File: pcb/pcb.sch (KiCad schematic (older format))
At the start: 70 parts, among them SW1 SW_PUSH, SW10 SW_PUSH, SW11 SW_PUSH, SW12 SW_PUSH, SW13 SW_PUSH, SW14 SW_PUSH, SW15 SW_PUSH, SW16 SW_PUSH, SW17 SW_PUSH, SW18 SW_PUSH, SW19 SW_PUSH, SW2 SW_PUSH, SW20 SW_PUSH, SW21 SW_PUSH, SW22 SW_PUSH, SW23 SW_PUSH, SW24 SW_PUSH, SW25 SW_PUSH, SW26 SW_PUSH, SW27 SW_PUSH, SW28 SW_PUSH, SW29 SW_PUSH, SW3 SW_PUSH, SW30 SW_PUSH, SW31 SW_PUSH, SW32 SW_PUSH, SW33 Rotary_Encoder_Switch, SW34 SW_PUSH, SW4 SW_PUSH, SW5 SW_PUSH, SW6 SW_PUSH, SW7 SW_PUSH, SW8 SW_PUSH, SW9 SW_PUSH, U1 ProMicro

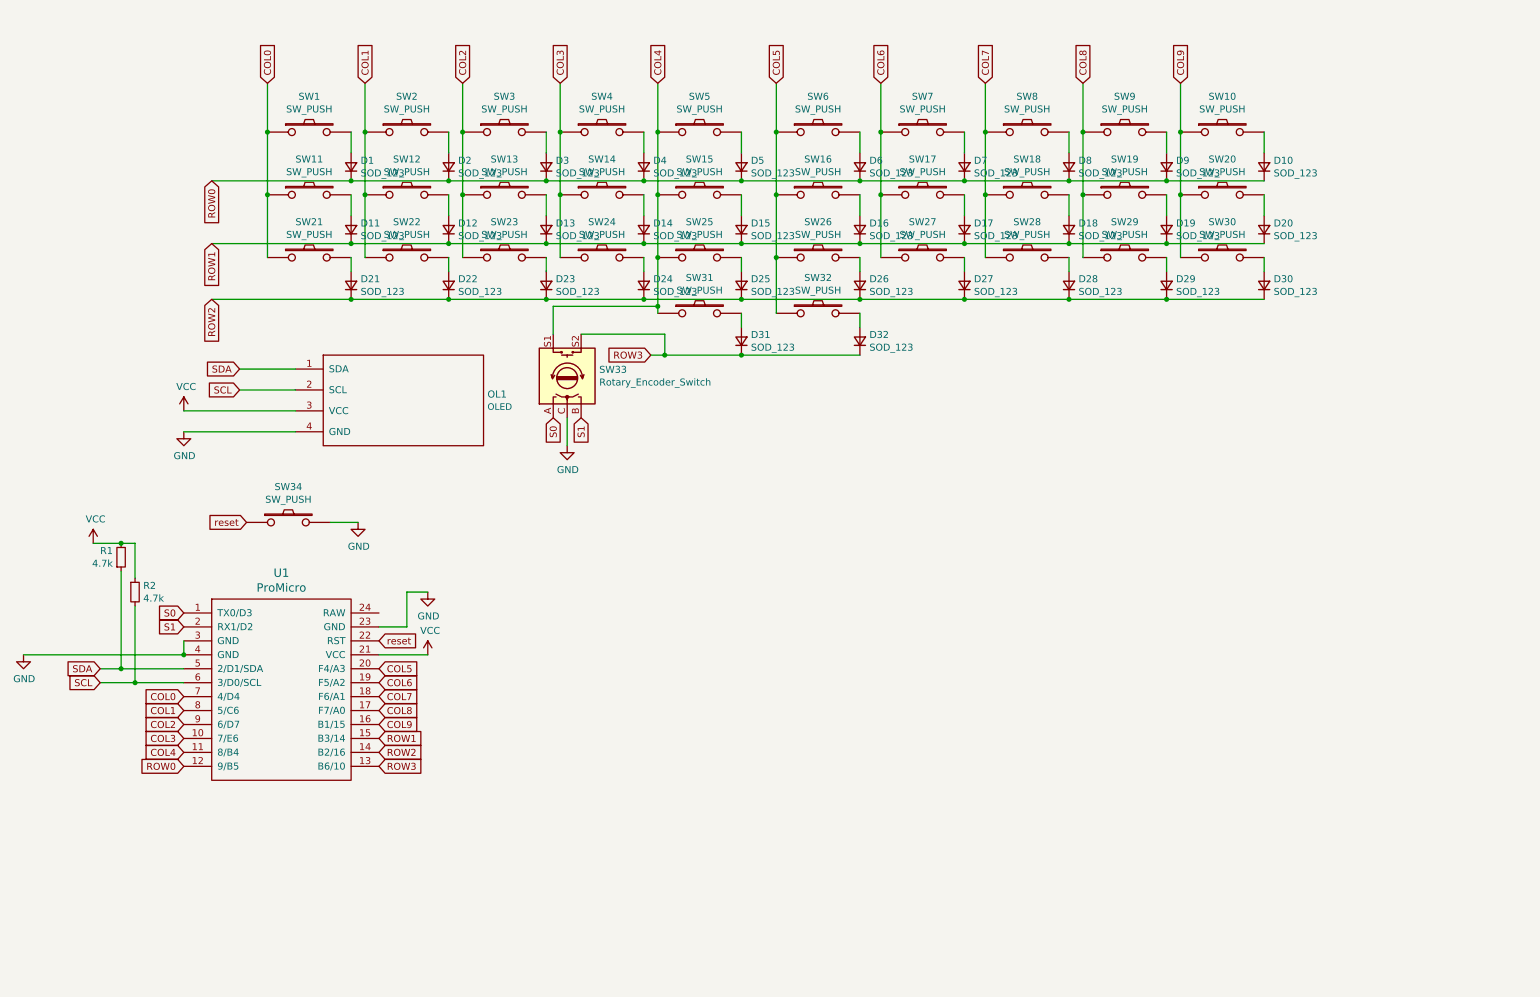
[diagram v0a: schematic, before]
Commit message: Major updates
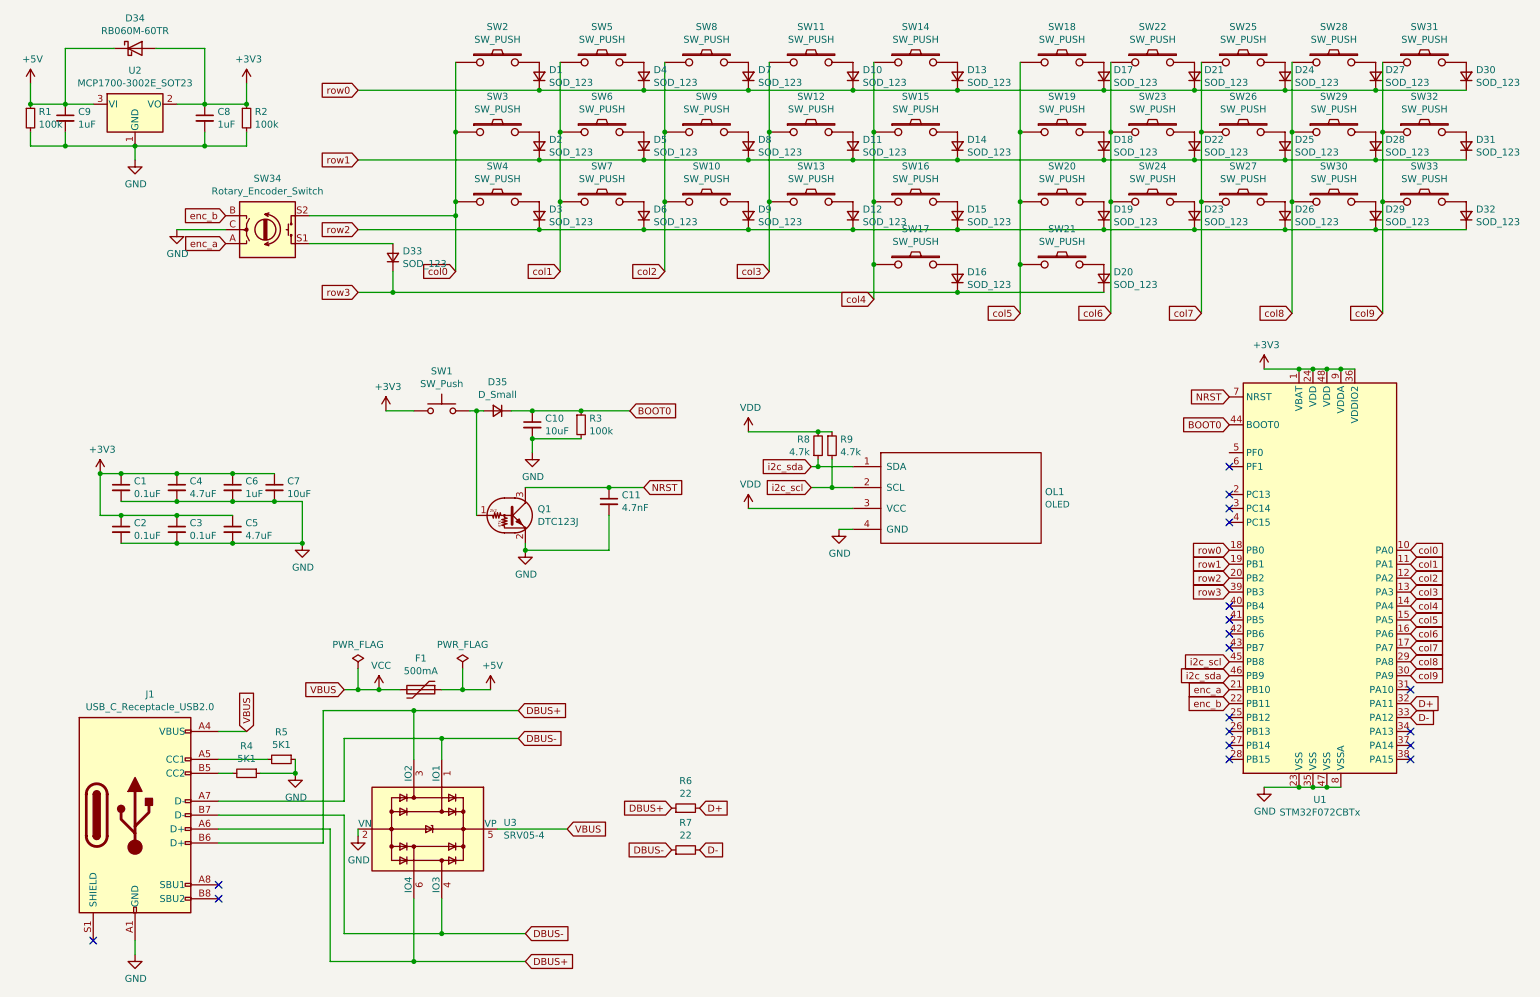
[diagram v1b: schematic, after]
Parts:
- removed SW1: SW_PUSH, MX_Only:MXOnly-1U-NoLED, symbol kbd:SW_PUSH
- removed SW33: Rotary_Encoder_Switch, keebio-parts:RotaryEncoder_EC11, symbol Device:Rotary_Encoder_Switch
- removed SW34: SW_PUSH, kbd:ResetSW_1side, symbol kbd:SW_PUSH
- removed U1: ProMicro, kbd:ProMicro_v3.5, symbol kbd:ProMicro
- added C1, C2, C3: 0.1uF, Capacitor_SMD:C_0805_2012Metric, symbol Device:C_Small
- added C10, C7: 10uF, Capacitor_SMD:C_0805_2012Metric, symbol Device:C_Small
- added C11: 4.7nF, Capacitor_SMD:C_0805_2012Metric, symbol Device:C_Small
- added C4, C5: 4.7uF, Capacitor_SMD:C_0805_2012Metric, symbol Device:C_Small
- added C6, C8, C9: 1uF, Capacitor_SMD:C_0805_2012Metric, symbol Device:C_Small
- added D33: SOD_123, Diode_SMD:D_SOD-123, symbol Device:D_Small
- added D34: RB060M-60TR, Diode_SMD:D_SOD-123, symbol Device:D_Schottky
- added D35: D_Small, Diode_SMD:D_SOD-123, symbol Device:D_Small
- added F1: 500mA, Fuse:Fuse_1206_3216Metric, symbol Device:Polyfuse
- added J1: USB_C_Receptacle_USB2.0, Connector_USB:USB_C_Receptacle_HRO_TYPE-C-31-M-12, symbol Connector:USB_C_Receptacle_USB2.0
- added Q1: DTC123J, Package_TO_SOT_SMD:SOT-23, symbol Transistor_BJT:DTC123J
- added R3: 100k, Resistor_SMD:R_0805_2012Metric, symbol Device:R_Small
- added R4, R5: 5K1, Resistor_SMD:R_0805_2012Metric, symbol Device:R_Small
- added R6, R7: 22, Resistor_SMD:R_0805_2012Metric, symbol Device:R_Small
- added R8, R9: 4.7k, Resistor_SMD:R_0805_2012Metric, symbol Device:R_Small
- added SW1: SW_Push, kbd:ResetSW, symbol Switch:SW_Push
- added SW33: SW_PUSH, MX_Only:MXOnly-1U-NoLED, symbol kbd:SW_PUSH
- added SW34: Rotary_Encoder_Switch, keebio-parts:RotaryEncoder_Alps_EC11E-Switch_Vertical_H20mm, symbol Device:Rotary_Encoder_Switch
- added U1: STM32F072CBTx, Package_QFP:LQFP-48_7x7mm_P0.5mm, symbol MCU_ST_STM32F0:STM32F072CBTx
- added U2: MCP1700-3002E_SOT23, Package_TO_SOT_SMD:SOT-23, symbol Regulator_Linear:MCP1700-3002E_SOT23
- added U3: SRV05-4, Package_TO_SOT_SMD:SOT-23-6, symbol Power_Protection:SRV05-4
- D1, D10, D11, D12, D13, D14, D15, D16, D17, D18, D19, D2, D20, D21, D22, D23, D24, D25, D26, D27, D28, D29, D3, D30, D31, D32, D4, D5, D6, D7, D8, D9: footprint kbd:D3_TH -> Diode_SMD:D_SOD-123
- OL1: footprint kbd:OLED_1side -> kbd:OLED
- R1, R2: value 4.7k -> 100k; footprint Resistor_THT:R_Axial_DIN0204_L3.6mm_D1.6mm_P1.90mm_Vertical -> Resistor_SMD:R_0805_2012Metric
- SW17, SW21: footprint MX_Only:MXOnly-1U-NoLED -> MX_Only:MXOnly-2U-NoLED
- SW31, SW32: footprint MX_Only:MXOnly-2U-NoLED -> MX_Only:MXOnly-1U-NoLED
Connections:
- net GND: now also R1.2, R2.2, C1.2, C10.2, C11.2, C2.2, C3.2, C4.2, C5.2, C6.2, C7.2, C8.2, C9.2, J1.A1 (GND), J1.A12 (GND), J1.B1 (GND), J1.B12 (GND), Q1.2 (E), R3.2, R4.1, R5.1, SW34.C, U1.23 (VSS), U1.35 (VSS), U1.47 (VSS), U1.8 (VSSA), U2.1 (GND), U3.2 (VN)
- net VCC: now also F1.2, J1.A4 (VBUS), J1.A9 (VBUS), J1.B4 (VBUS), J1.B9 (VBUS), U3.5 (VP); no longer OL1.3 (VCC), R1.2, R2.1
- net at D1.2 (A): now also SW2.2
- net at SW11.2: now also D10.2 (A); no longer D11.2 (A)
- net at SW21.2: now also D20.2 (A); no longer D21.2 (A)
- net at D2.2 (A): now also SW3.2; no longer SW2.2
- net at SW12.2: now also D11.2 (A); no longer D12.2 (A)
- net at SW22.2: now also D21.2 (A); no longer D22.2 (A)
- net at SW23.2: now also D22.2 (A); no longer D23.2 (A)
- net at SW13.2: now also D12.2 (A); no longer D13.2 (A)
- net at D3.2 (A): now also SW4.2; no longer SW3.2
- net at D4.2 (A): now also SW5.2; no longer SW4.2
- net at SW14.2: now also D13.2 (A); no longer D14.2 (A)
- net at SW24.2: now also D23.2 (A); no longer D24.2 (A)
- net at SW25.2: now also D24.2 (A); no longer D25.2 (A)
- net at SW31.2: now also D30.2 (A); no longer D31.2 (A)
- net at SW32.2: now also D31.2 (A); no longer D32.2 (A)
- net at SW15.2: now also D14.2 (A); no longer D15.2 (A)
- net at D5.2 (A): now also SW6.2; no longer SW5.2
- net at D6.2 (A): now also SW7.2; no longer SW6.2
- net at SW16.2: now also D15.2 (A); no longer D16.2 (A)
- net at SW26.2: now also D25.2 (A); no longer D26.2 (A)
- net at SW27.2: now also D26.2 (A); no longer D27.2 (A)
- net at SW17.2: now also D16.2 (A); no longer D17.2 (A)
- net at D7.2 (A): now also SW8.2; no longer SW7.2
- net at D8.2 (A): now also SW9.2; no longer SW8.2
- net at SW18.2: now also D17.2 (A); no longer D18.2 (A)
- net at SW28.2: now also D27.2 (A); no longer D28.2 (A)
- net at SW29.2: now also D28.2 (A); no longer D29.2 (A)
- net at SW30.2: now also D29.2 (A); no longer D30.2 (A)
- net at SW19.2: now also D18.2 (A); no longer D19.2 (A)
- net at D9.2 (A): now also SW10.2; no longer SW9.2
- net at SW20.2: now also D19.2 (A); no longer D20.2 (A)
- net COL0 renamed col3
- net col3: now also SW12.1, SW13.1, U1.13 (PA3); no longer SW21.1
- removed net COL1: SW12.1, SW2.1, SW22.1
- removed net COL2: SW13.1, SW23.1, SW3.1
- removed net COL3: SW14.1, SW24.1, SW4.1
- removed net COL4: SW15.1, SW25.1, SW31.1, SW5.1
- removed net COL5: SW16.1, SW26.1, SW32.1, SW6.1
- removed net COL6: SW17.1, SW27.1, SW7.1
- removed net COL7: SW18.1, SW28.1, SW8.1
- removed net COL8: SW19.1, SW29.1, SW9.1
- removed net COL9: SW10.1, SW20.1, SW30.1
- removed net ROW0: D1.1 (K), D10.1 (K), D2.1 (K), D3.1 (K), D4.1 (K), D5.1 (K), D6.1 (K), D7.1 (K), D8.1 (K), D9.1 (K)
- removed net ROW1: D11.1 (K), D12.1 (K), D13.1 (K), D14.1 (K), D15.1 (K), D16.1 (K), D17.1 (K), D18.1 (K), D19.1 (K), D20.1 (K)
- removed net ROW2: D21.1 (K), D22.1 (K), D23.1 (K), D24.1 (K), D25.1 (K), D26.1 (K), D27.1 (K), D28.1 (K), D29.1 (K), D30.1 (K)
- net ROW3 renamed row1
- net row1: now also D11.1 (K), D14.1 (K), D18.1 (K), D2.1 (K), D22.1 (K), D25.1 (K), D28.1 (K), D5.1 (K), D8.1 (K), U1.19 (PB1); no longer D32.1 (K)
- net SCL renamed i2c_scl
- net i2c_scl: now also R9.2, U1.45 (PB8); no longer R2.2
- net SDA renamed +5V
- net +5V: now also C9.1, D34.1 (K), F1.1, U2.3 (VI); no longer OL1.1 (SDA)
- new net: J1.A5 (CC1), R5.2
- new net: J1.B5 (CC2), R4.2
- new net: D35.2 (A), Q1.1 (B), SW1.2
- new net: D32.2 (A), SW33.2
- new net: D33.2 (A), SW34.S1
- new net +3V3: C1.1, C2.1, C3.1, C4.1, C5.1, C6.1, C7.1, C8.1, D34.2 (A), R2.1, SW1.1, U1.1 (VBAT), U1.24 (VDD), U1.36 (VDDIO2), U1.48 (VDD), U1.9 (VDDA), U2.2 (VO)
- new net BOOT0: C10.1, D35.1 (K), R3.1, U1.44 (BOOT0)
- new net D+: R6.2, U1.32 (PA11)
- new net D-: R7.2, U1.33 (PA12)
- new net DBUS+: J1.A6 (D+), J1.B6 (D+), R6.1, U3.3 (IO2), U3.6 (IO4)
- new net DBUS-: J1.A7 (D-), J1.B7 (D-), R7.1, U3.1 (IO1), U3.4 (IO3)
- new net NRST: C11.1, Q1.3 (C), U1.7 (NRST)
- new net VDD: OL1.3 (VCC), R8.2, R9.1
- new net col0: SW2.1, SW3.1, SW34.S2, SW4.1, U1.10 (PA0)
- new net col1: SW5.1, SW6.1, SW7.1, U1.11 (PA1)
- new net col2: SW10.1, SW8.1, SW9.1, U1.12 (PA2)
- new net col4: SW14.1, SW15.1, SW16.1, SW17.1, U1.14 (PA4)
- new net col5: SW18.1, SW19.1, SW20.1, SW21.1, U1.15 (PA5)
- new net col6: SW22.1, SW23.1, SW24.1, U1.16 (PA6)
- new net col7: SW25.1, SW26.1, SW27.1, U1.17 (PA7)
- new net col8: SW28.1, SW29.1, SW30.1, U1.29 (PA8)
- new net col9: SW31.1, SW32.1, SW33.1, U1.30 (PA9)
- new net enc_a: SW34.A, U1.21 (PB10)
- new net enc_b: SW34.B, U1.22 (PB11)
- new net i2c_sda: OL1.1 (SDA), R8.1, U1.46 (PB9)
- new net row0: D1.1 (K), D10.1 (K), D13.1 (K), D17.1 (K), D21.1 (K), D24.1 (K), D27.1 (K), D30.1 (K), D4.1 (K), D7.1 (K), U1.18 (PB0)
- new net row2: D12.1 (K), D15.1 (K), D19.1 (K), D23.1 (K), D26.1 (K), D29.1 (K), D3.1 (K), D32.1 (K), D6.1 (K), D9.1 (K), U1.20 (PB2)
- new net row3: D16.1 (K), D20.1 (K), D33.1 (K), U1.39 (PB3)
- no-connect marks 0 -> 19
